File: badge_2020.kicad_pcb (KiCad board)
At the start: 2 copper layers, 105.7 x 83.3 mm, 27 parts, among them J1 USB_A, Q1 AOI409, SW1 SW_Push, SW2 SW, U1 ATTINY85-20PU

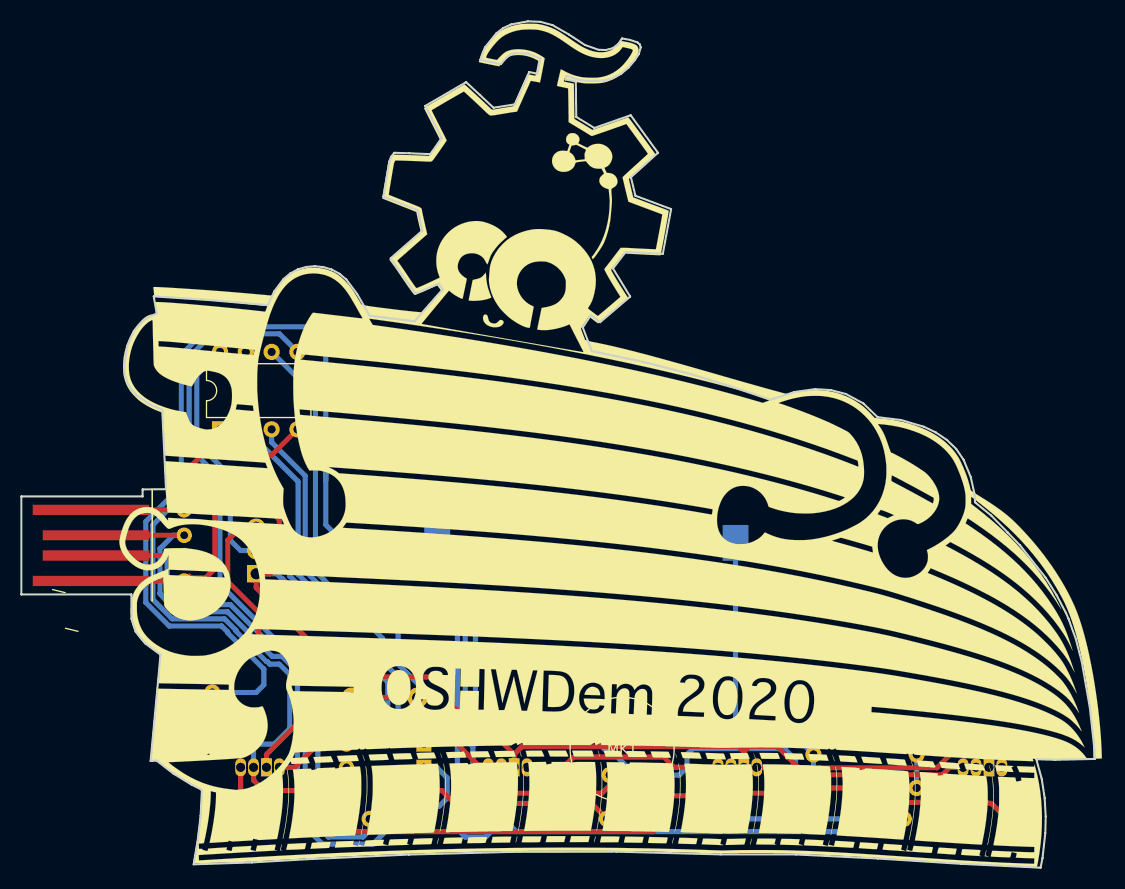
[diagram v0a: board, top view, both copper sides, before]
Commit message: Retoques menores
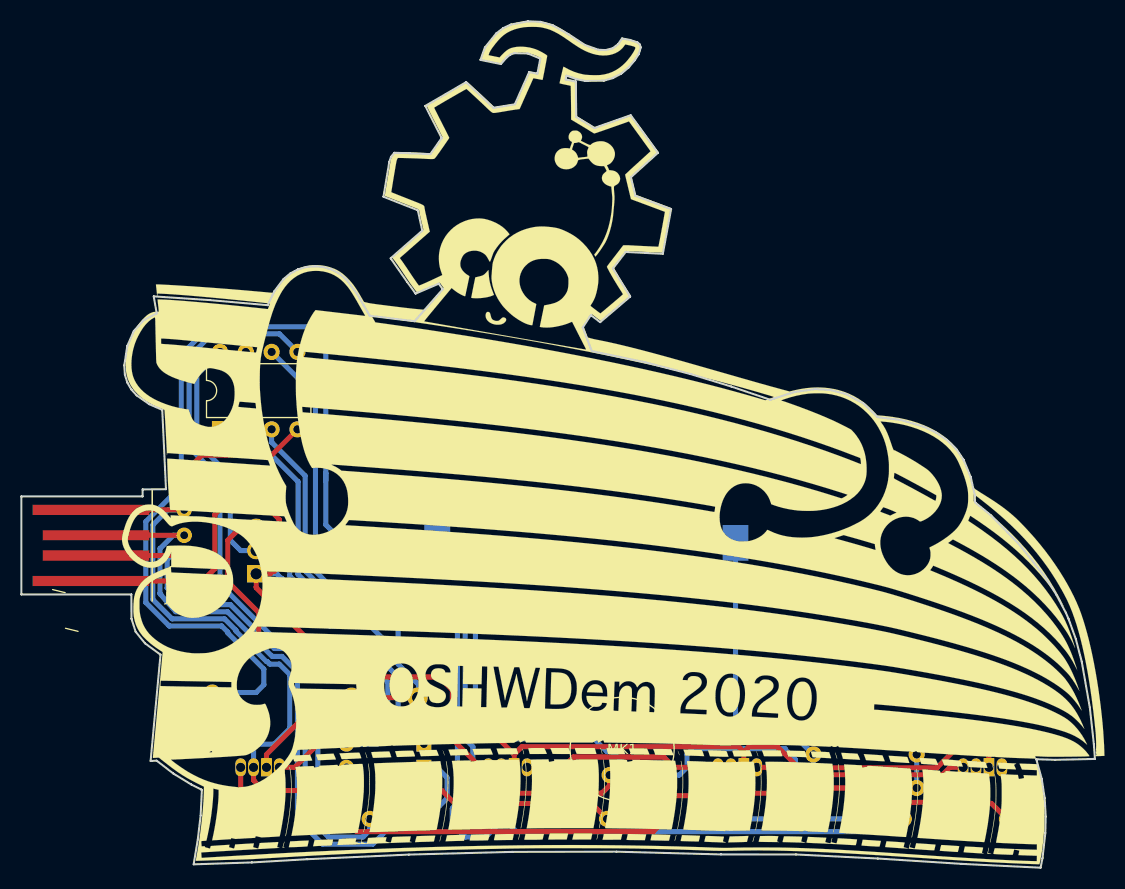
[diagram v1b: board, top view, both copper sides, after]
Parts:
- removed the G*** at (330.2, 211.3)
- moved G*** 0.36 mm to (175.8, 107.4)
